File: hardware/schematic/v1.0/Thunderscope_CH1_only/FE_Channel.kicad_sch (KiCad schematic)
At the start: 105 parts, among them J1 Conn_Coaxial, J3_1 UFL, J4_1 UFL, K1000_1 G6K-2F-RF, K1001_1 G6K-2F-RF, Q1002_1 DMN62D0UW, Q1003_1 DMN62D0UW, U1001_1 TMUX4053, U1008_1 LMH6518, U1009_1 BUF802, U1011_1 OPA140AIDBVR

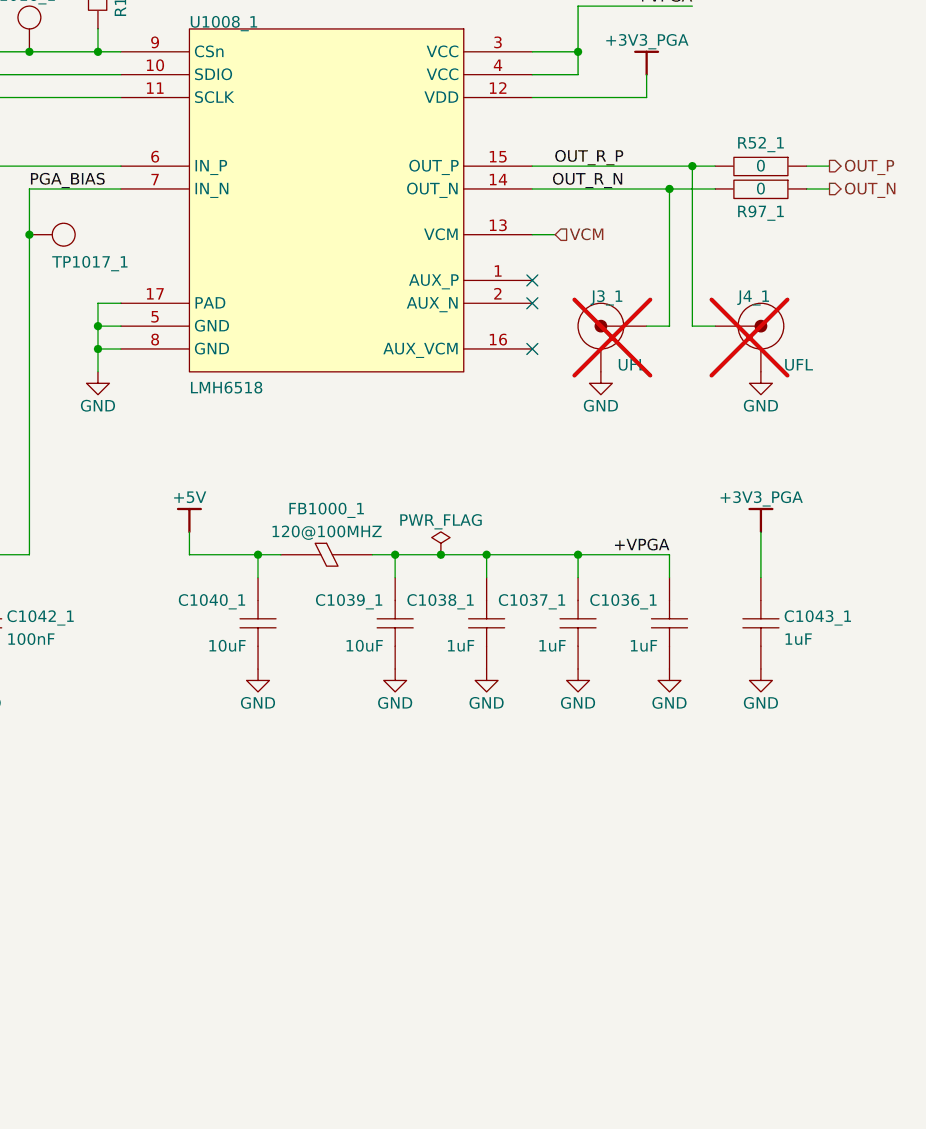
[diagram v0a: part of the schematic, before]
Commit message: sch update
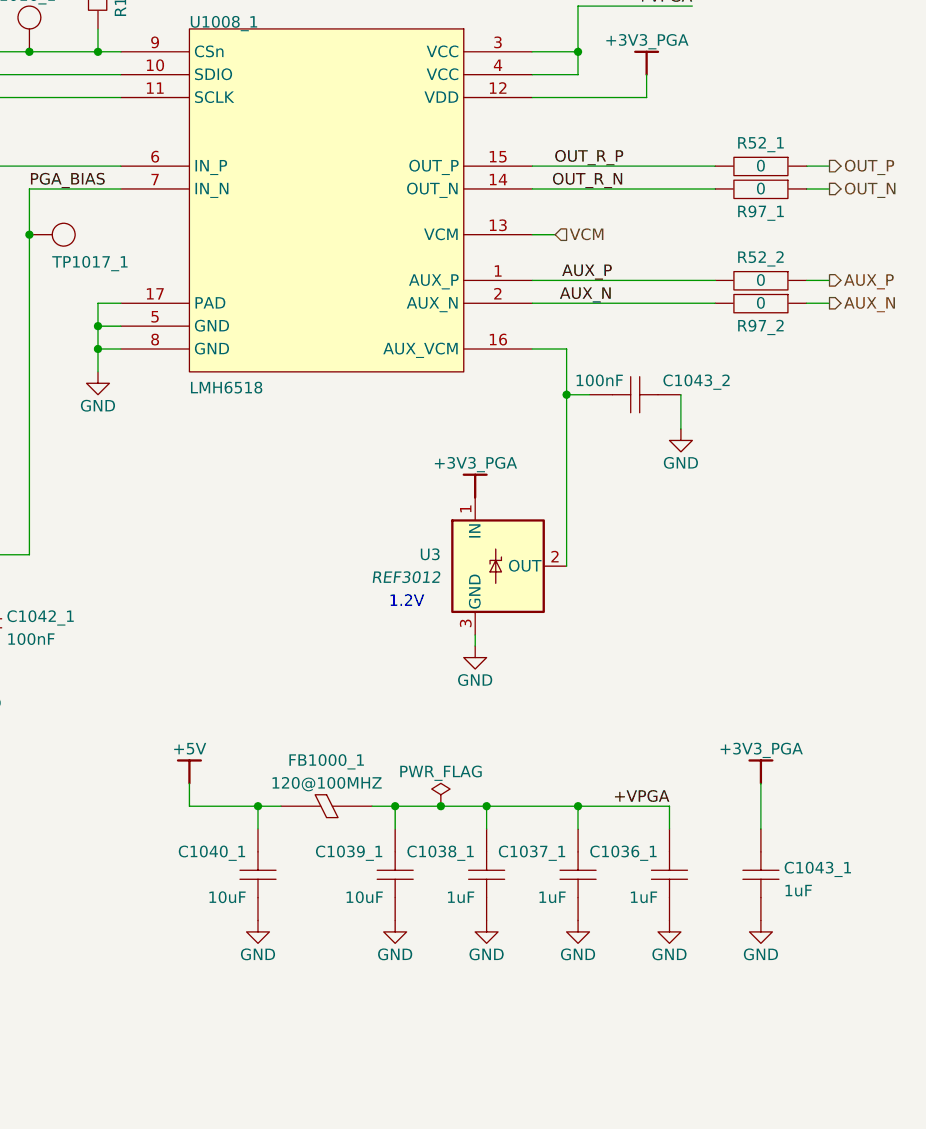
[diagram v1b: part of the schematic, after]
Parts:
- removed J3_1, J4_1: UFL, Thunderscope_Rev5:TE_2334884-1, symbol Thunderscope_Rev5:UFL Jack SMD
- added C1043_2: 100nF, Thunderscope_Rev5:GEN_C_0402, symbol Thunderscope_Rev5:CAP 1uF 25V X5R 0402
- added R52_2, R97_2: 0, Thunderscope_Rev5:GEN_R_0402, symbol Thunderscope_Rev5:RES 0 OHM 1/16W 0402
- added U3: REF3012, Package_TO_SOT_SMD:SOT-23, symbol Reference_Voltage:REF3012
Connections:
- net +3V3_PGA: now also U3.1 (IN)
- net GND: now also C1043_2.2, U3.3 (GND)
- net AUX_P: now reaches U1008_1.1 (AUX_P)
- net AUX_P: now also R52_2.1, R52_2.2
- net at U1008_1.16 (AUX_VCM): now also C1043_2.1, U3.2 (OUT)
- net AUX_N: now reaches U1008_1.2 (AUX_N)
- net AUX_N: now also R97_2.1, R97_2.2
- no-connect marks 4 -> 1
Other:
- note added: "1.2V"
- moved on the sheet: C1036_1, C1037_1, C1038_1, C1039_1, C1040_1, C1043_1, FB1000_1
